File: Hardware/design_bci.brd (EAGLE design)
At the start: 182.6 x 115.6 mm, 12 parts, among them IC1 AD623N

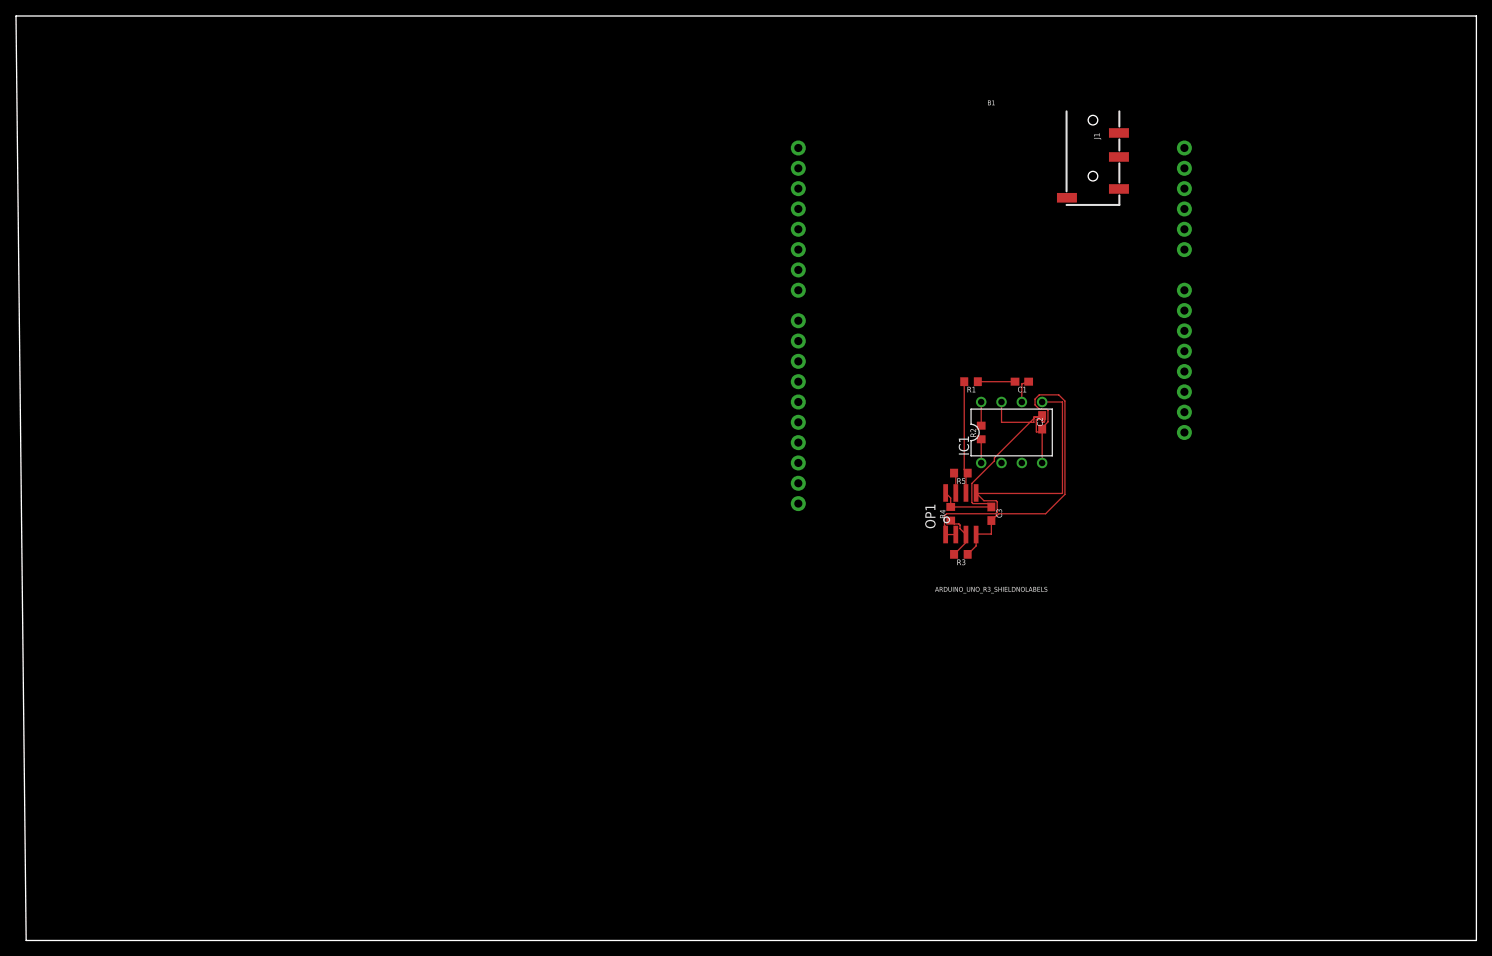
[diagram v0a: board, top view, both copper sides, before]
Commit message: updated
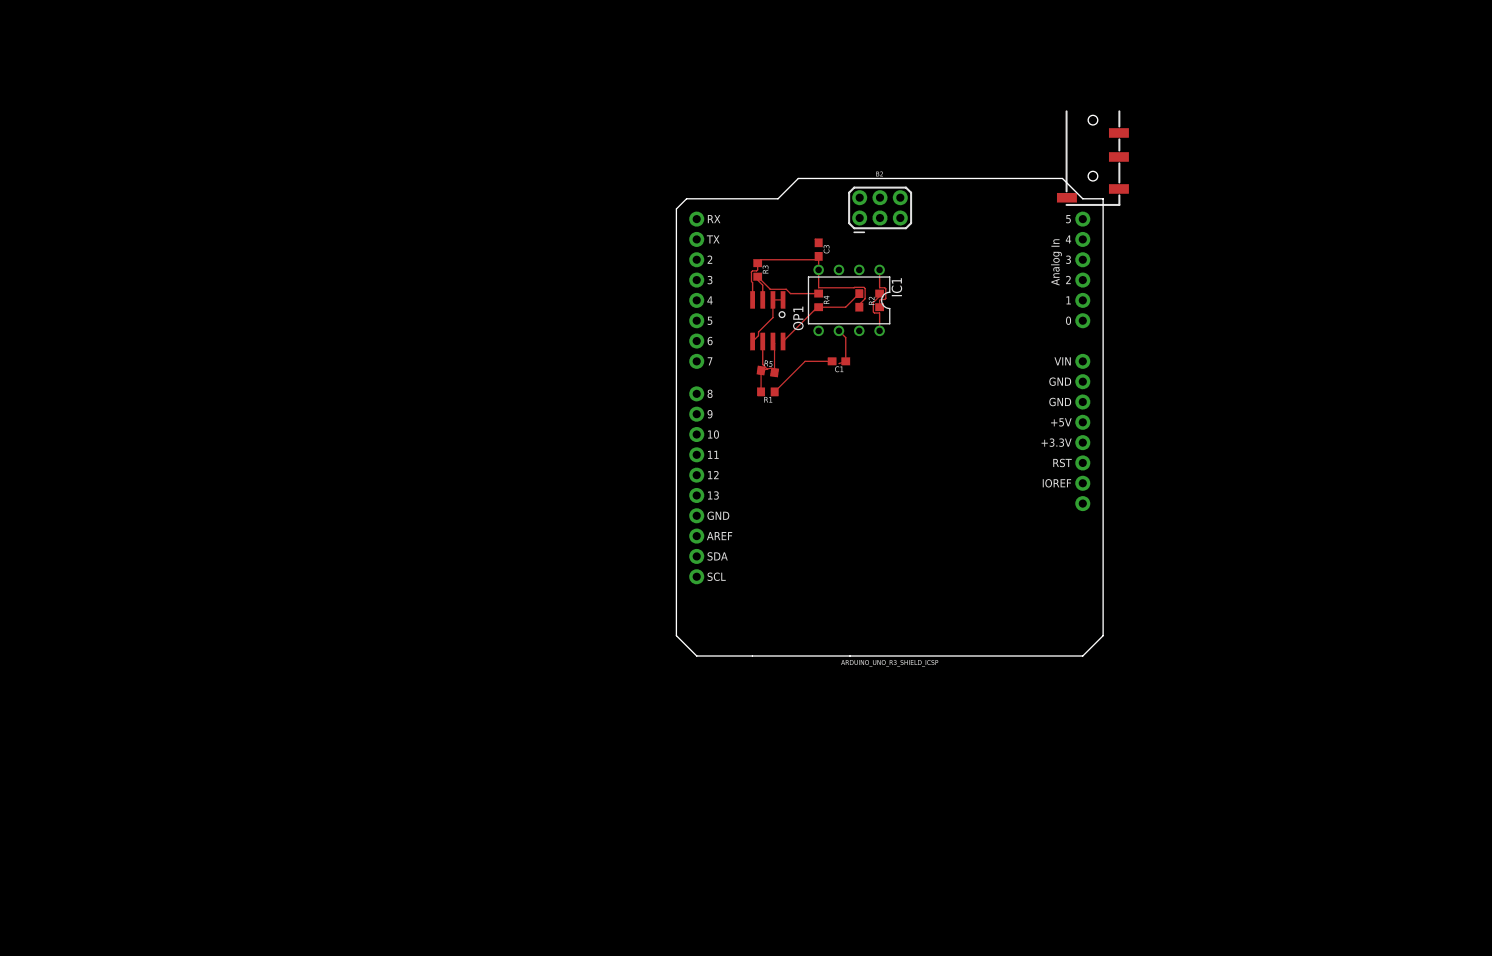
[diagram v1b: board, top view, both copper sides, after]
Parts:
- removed B1: ARDUINO_UNO_R3_SHIELDNOLABELS, LinnesLab-Microcontrollers:UNO_R3_SHIELD_NOLABELS
- added B2: ARDUINO_UNO_R3_SHIELD_ICSP, LinnesLab-Microcontrollers:UNO_R3_SHIELD_ICSP
- moved R3 43.7 mm to (10.2, 48.3), turned to 270 degrees
- moved C3 39.5 mm to (17.8, 50.8)
- moved OP1 34.1 mm to (11.4, 41.9), turned to 180 degrees
- moved R4 31.4 mm to (17.8, 44.5), turned to 270 degrees
- moved C2 27.5 mm to (22.9, 44.5)
- moved R5 27.3 mm to (11.4, 35.6), turned to 351.8 degrees
- moved IC1 26.2 mm to (21.6, 44.5), turned to 180 degrees
- moved R1 25.4 mm to (11.4, 33.0)
- moved C1 23.0 mm to (20.3, 36.8)
- moved R2 20.8 mm to (25.4, 44.5)
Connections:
- new net N$10: IC1.2, J1.LEFT
- new net N$9: IC1.3, J1.RIGHT
- net GND: now also J1.GND, J1.GND/MIC
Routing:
- net N$6: track 39.6 -> 7.52 mm
- net 3.3V: track 35.8 -> 12.6 mm
- net GND: track 45.6 -> 25.5 mm
- net N$7: track 14.2 -> 7.64 mm
- net N$3: track 5.99 -> 11.2 mm
- net N$5: track 4.65 -> 8.77 mm
- net N$2: track 2.96 -> 5.99 mm
- net N$1: track 2.96 -> 5.68 mm
- net N$4: track 3.15 -> 5.06 mm
- net N$8: track 2.57 -> 3.96 mm
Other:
- board size 182.6 x 115.6 mm -> 53.3 x 59.7 mm
